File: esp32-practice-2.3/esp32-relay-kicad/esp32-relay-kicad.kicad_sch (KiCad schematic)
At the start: 6 parts, among them M1 Motor_DC, Q1 PN2222A, U1 YD-ESP32-S3

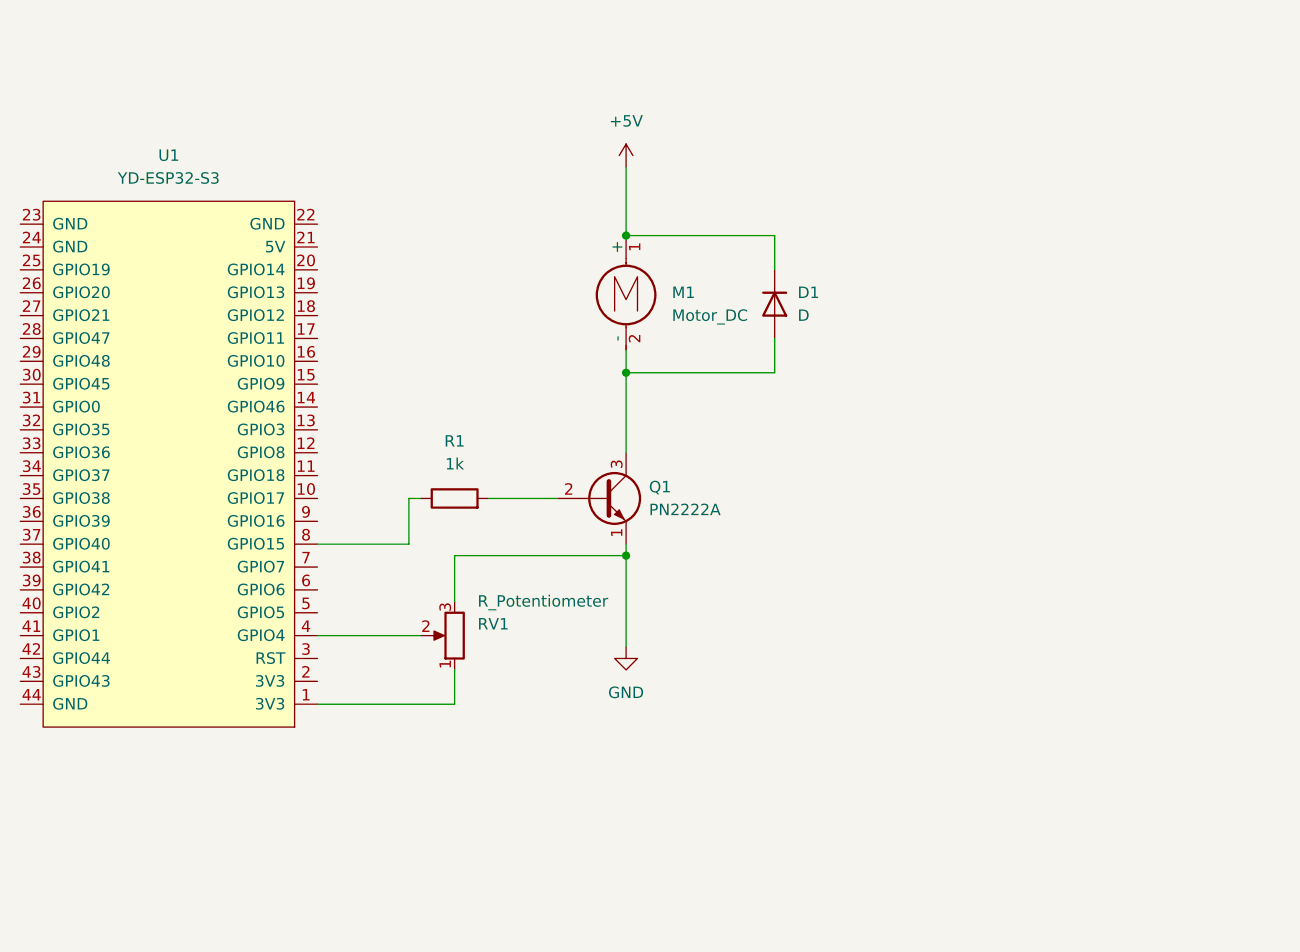
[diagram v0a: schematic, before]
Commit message: 2.5 timers homework
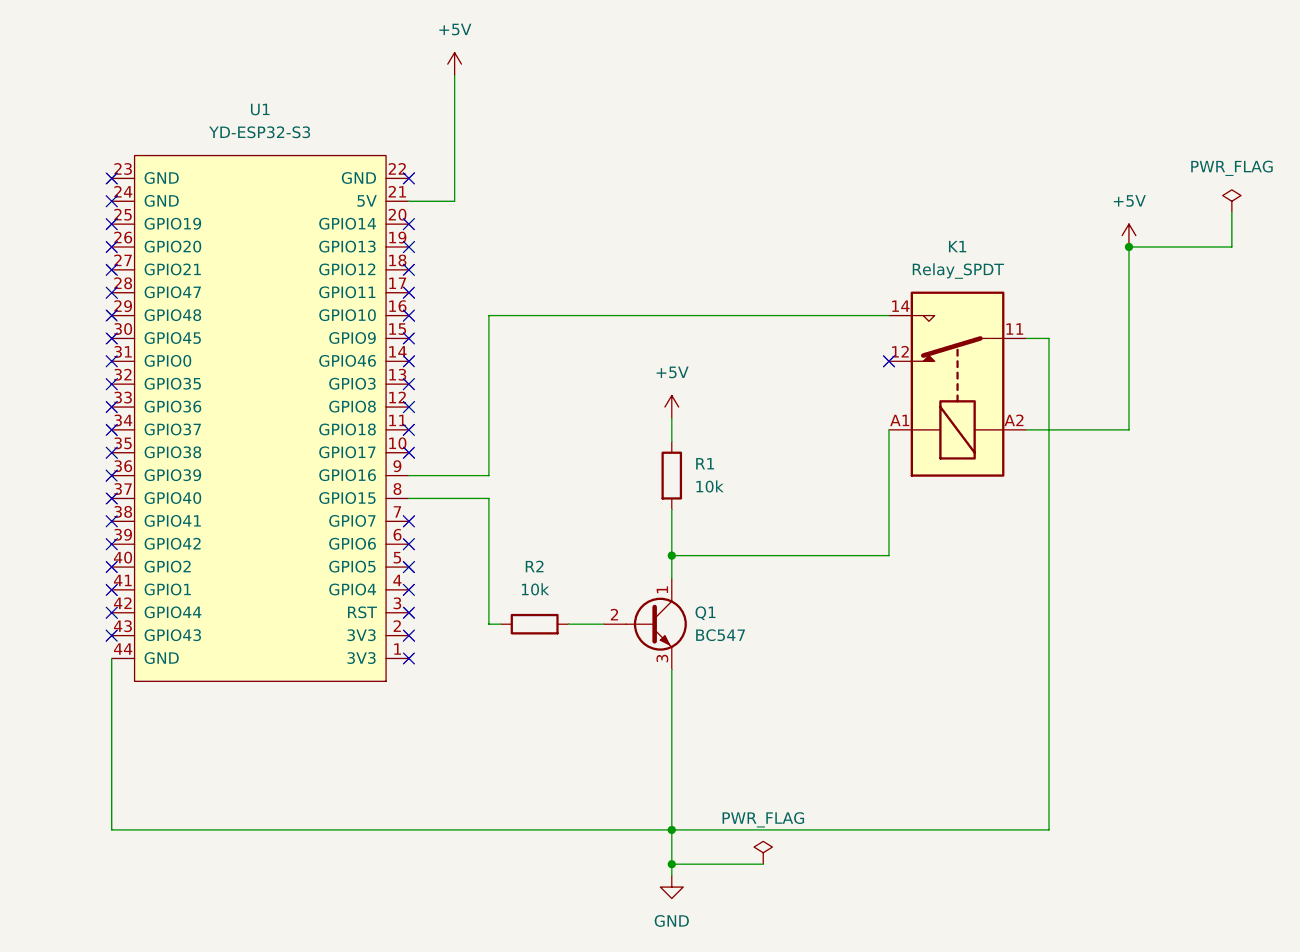
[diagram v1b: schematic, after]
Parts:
- removed D1: D, symbol Device:D
- removed M1: Motor_DC, symbol Motor:Motor_DC
- removed Q1: PN2222A, Package_TO_SOT_THT:TO-92_Inline, symbol Transistor_BJT:PN2222A
- removed RV1: R_Potentiometer, symbol Device:R_Potentiometer
- added K1: Relay_SPDT, symbol Relay:Relay_SPDT
- added Q1: BC547, Package_TO_SOT_THT:TO-92_Inline, symbol Transistor_BJT:BC547
- added R2: 10k, symbol Device:R
- R1: value 1k -> 10k
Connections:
- net +5V: now also R1.1, U1.21 (5V), K1.A2
- net GND: now also U1.44 (GND), K1.11, Q1.3 (E)
- net at U1.8 (GPIO15): now also R2.1; no longer R1.1
- net at U1.9 (GPIO16): now also K1.14
- net at R1.2: now also K1.A1, Q1.1 (C)
- new net: Q1.2 (B), R2.2
- no-connect marks 0 -> 41
